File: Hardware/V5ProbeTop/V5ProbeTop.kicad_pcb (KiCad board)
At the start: 2 copper layers, 126.4 x 15.2 mm, 38 parts, among them J1 Conn_01x13_Socket, J2 Conn_01x13_Socket

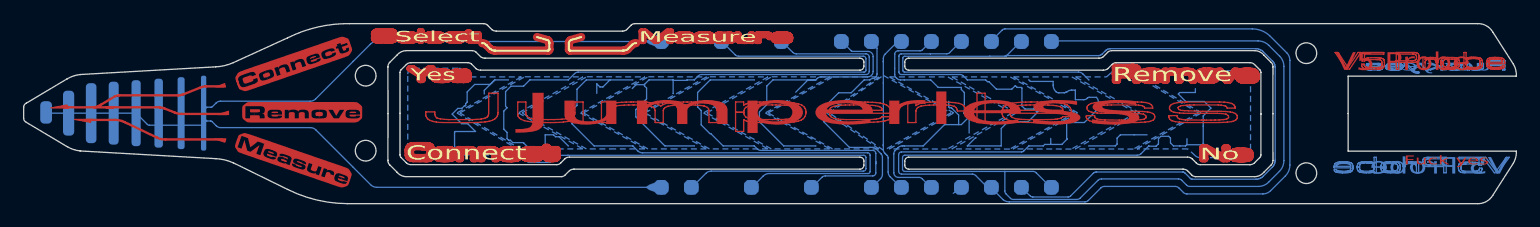
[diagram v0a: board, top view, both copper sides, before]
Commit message: Add post campaign update draft
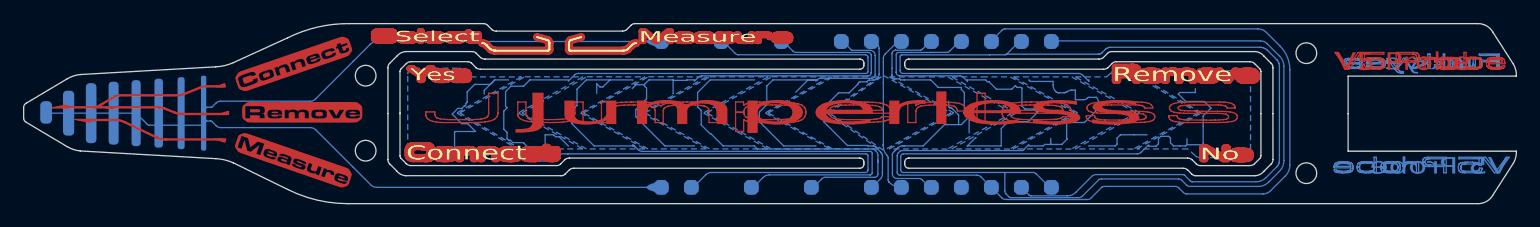
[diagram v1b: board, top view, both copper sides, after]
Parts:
- moved TP7 0.26 mm to (144.1, 88.9)
- moved TP21 0.26 mm to (144.1, 83.5)
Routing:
- net Net-(J1-Pin_3): track 88.6 -> 90.3 mm
- net Net-(J1-Pin_12): track 49.4 -> 50.3 mm
- net Net-(J1-Pin_6): track 31.0 -> 31.8 mm
- net Net-(J1-Pin_9): track 25.1 -> 25.9 mm
- net Net-(J1-Pin_11): track 40.3 -> 40.9 mm
- net Net-(J1-Pin_14): track 65.9 -> 66.5 mm
- net Net-(J1-Pin_13): track 56.7 -> 57.3 mm
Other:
- outline, holes or cut-outs redrawn
